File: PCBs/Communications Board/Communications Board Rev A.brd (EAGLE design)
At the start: 95.9 x 90.2 mm, 21 parts

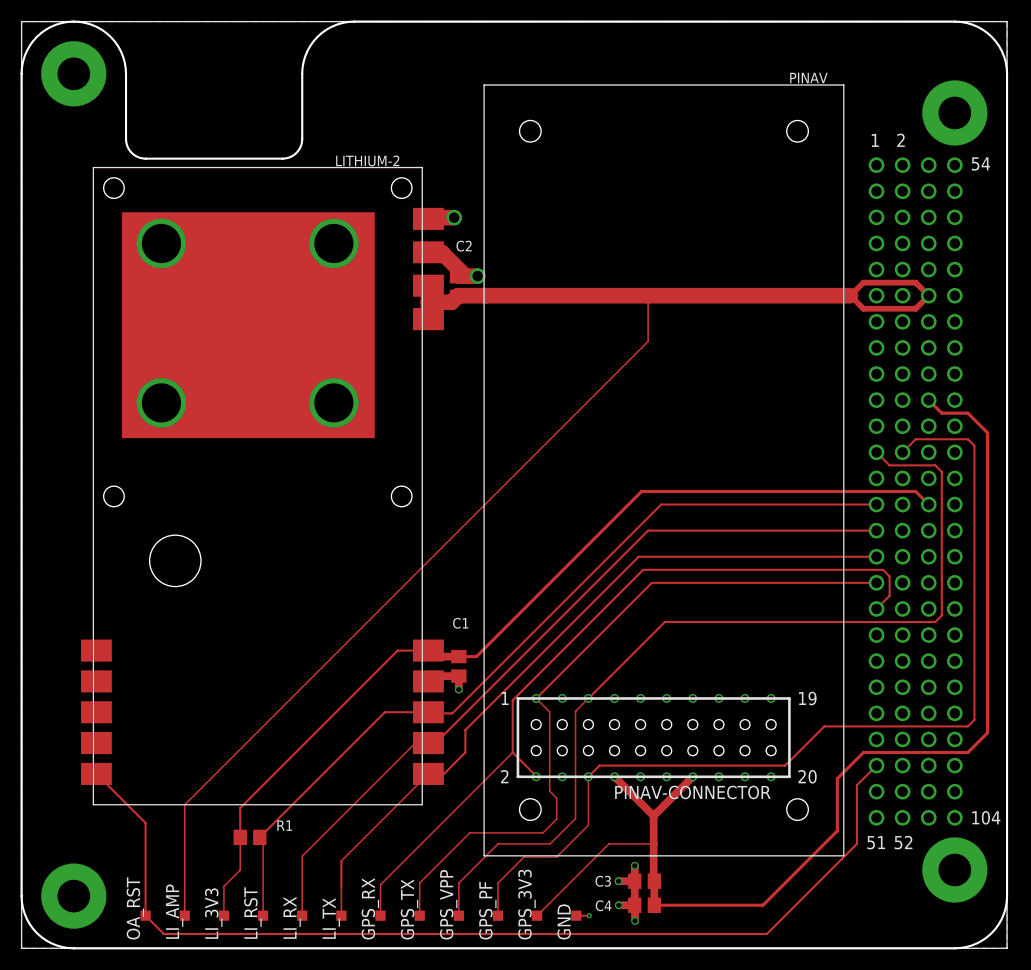
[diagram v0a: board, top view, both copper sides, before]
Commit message: Rev A2
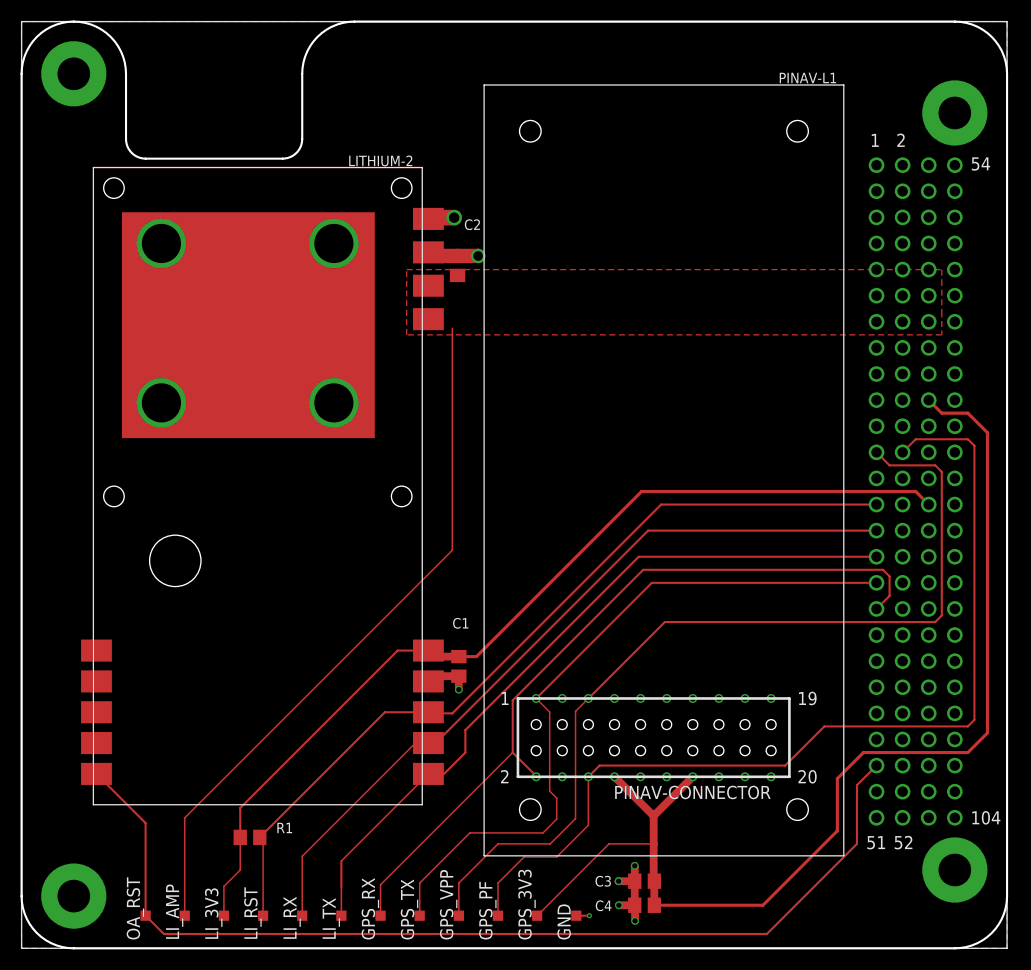
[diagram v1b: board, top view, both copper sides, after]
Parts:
- moved C2 2.03 mm to (42.4, 66.4)
- renumbered PINAV to PINAV-L1
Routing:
- net SW3: track 141.5 -> 67.9 mm
- net GND: track 23.8 -> 22.5 mm
- added copper zone on layer 1, net SW3
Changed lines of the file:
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@@
 <attribute name="VALUE" x="41.275" y="29.845" size="1.016" layer="27"/>
 </element>
-<element name="C2" library="resistor" library_urn="urn:adsk.eagle:library:348" package="C0805" package3d_urn="urn:adsk.eagle:package:23617/2" value="47uF" x="42.418" y="64.389" smashed="yes" rot="R90">
-<attribute name="NAME" x="43.9166" y="68.834" size="1.016" layer="25" rot="R180"/>
-<attribute name="VALUE" x="44.7548" y="67.564" size="1.016" layer="27" rot="R180"/>
+<element name="C2" library="resistor" library_urn="urn:adsk.eagle:library:348" package="C0805" package3d_urn="urn:adsk.eagle:package:23617/2" value="47uF" x="42.418" y="66.421" smashed="yes" rot="R90">
+<attribute name="NAME" x="44.7294" y="70.9168" size="1.016" layer="25" rot="R180"/>
+<attribute name="VALUE" x="44.7548" y="69.596" size="1.016" layer="27" rot="R180"/>
 </element>
 <element name="C3" library="resistor" library_urn="urn:adsk.eagle:library:348" package="C0805" package3d_urn="urn:adsk.eagle:package:23617/2" value="0.1uF" x="60.613" y="6.531" smashed="yes" rot="R180">
@@
 <attribute name="VALUE" x="62.8564" y="3.6068" size="1.016" layer="27"/>
 </element>
-<element name="PINAV" library="Cubesat" package="PINAV-L1" value="" x="80" y="84" smashed="yes" rot="R180">
-<attribute name="NAME" x="74.6606" y="84.1734" size="1.016" layer="25"/>
+<element name="PINAV-L1" library="Cubesat" package="PINAV-L1" value="" x="80" y="84" smashed="yes" rot="R180">
+<attribute name="NAME" x="73.6446" y="84.1734" size="1.016" layer="25"/>
 </element>
 <element name="U$1" library="Cubesat" package="PC104_NO_DIMENSION" value="PC104_NO_DIMENSION" x="0" y="0"/>
@@
 </element>
 <element name="LITHIUM-2" library="Cubesat" package="LI-2" value="LI-2" x="6.985" y="13.97" smashed="yes">
-<attribute name="NAME" x="30.48" y="76.105" size="1.016" layer="25"/>
+<attribute name="NAME" x="31.75" y="76.105" size="1.016" layer="25"/>
 </element>
 <element name="LI_RST" library="testpad" library_urn="urn:adsk.eagle:library:385" package="TP10SQ" package3d_urn="urn:adsk.eagle:package:27962/1" value="TPSQTP10SQ" x="23.495" y="3.175" smashed="yes" rot="R90">
@@
 </element>
 <element name="R1" library="resistor" library_urn="urn:adsk.eagle:library:348" package="R0805" package3d_urn="urn:adsk.eagle:package:23553/2" value="47k" x="22.225" y="10.795" smashed="yes">
-<attribute name="NAME" x="24.765" y="11.43" size="1.016" layer="25"/>
-<attribute name="VALUE" x="24.765" y="9.525" size="1.016" layer="27"/>
+<attribute name="NAME" x="24.765" y="11.2014" size="1.016" layer="25"/>
+<attribute name="VALUE" x="24.765" y="9.8298" size="1.016" layer="27"/>
 </element>
 </elements>
@@
 <signal name="SW3">
 <contactref element="C2" pad="1"/>
-<wire x1="81.915" y1="64.77" x2="80.645" y2="63.5" width="0.5588" layer="1"/>
-<wire x1="81.915" y1="64.77" x2="86.995" y2="64.77" width="0.5588" layer="1"/>
-<wire x1="81.915" y1="62.23" x2="80.645" y2="63.5" width="0.5588" layer="1"/>
-<wire x1="81.915" y1="62.23" x2="86.995" y2="62.23" width="0.5588" layer="1"/>
-<wire x1="80.645" y1="63.5" x2="60.96" y2="63.5" width="1.524" layer="1"/>
 <contactref element="U$1" pad="63"/>
-<wire x1="86.995" y1="64.77" x2="88.265" y2="63.5" width="0.5588" layer="1"/>
-<wire x1="86.995" y1="62.23" x2="88.265" y2="63.5" width="0.5588" layer="1"/>
 <contactref element="LI_AMP" pad="TP"/>
-<wire x1="60.96" y1="63.5" x2="60.96" y2="59.055" width="0.1524" layer="1"/>
-<wire x1="15.875" y1="13.97" x2="15.875" y2="3.175" width="0.1524" layer="1"/>
-<wire x1="60.96" y1="59.055" x2="15.875" y2="13.97" width="0.1524" layer="1"/>
-<wire x1="45.151" y1="63.5" x2="60.96" y2="63.5" width="1.524" layer="1"/>
 <contactref element="LITHIUM-2" pad="V_AMP2"/>
 <contactref element="LITHIUM-2" pad="V_AMP1"/>
-<wire x1="39.784" y1="61.021" x2="39.585" y2="61.22" width="1.524" layer="1"/>
-<wire x1="45.151" y1="63.5" x2="45.151" y2="63.5" width="1.524" layer="1"/>
-<wire x1="42.418" y1="63.439" x2="42.479" y2="63.5" width="1.524" layer="1"/>
-<wire x1="42.479" y1="63.5" x2="45.151" y2="63.5" width="1.524" layer="1"/>
-<wire x1="39.585" y1="64.47" x2="39.585" y2="62.865" width="1.524" layer="1"/>
-<wire x1="39.585" y1="62.865" x2="39.585" y2="61.22" width="1.524" layer="1"/>
-<wire x1="39.585" y1="61.22" x2="39.784" y2="61.021" width="1.524" layer="1"/>
-<wire x1="39.585" y1="62.865" x2="41.844" y2="62.865" width="1.524" layer="1"/>
-<wire x1="41.844" y1="62.865" x2="42.418" y2="63.439" width="1.524" layer="1"/>
+<polygon width="0.1524" layer="1" thermals="no">
+<vertex x="89.535" y="65.024"/>
+<vertex x="89.535" y="61.976"/>
+<vertex x="89.535" y="59.69"/>
+<vertex x="37.465" y="59.69"/>
+<vertex x="37.465" y="66.04"/>
+<vertex x="89.535" y="66.04"/>
+</polygon>
+<wire x1="15.875" y1="3.175" x2="15.875" y2="12.7" width="0.1524" layer="1"/>
+<wire x1="15.875" y1="12.7" x2="41.91" y2="38.735" width="0.1524" layer="1"/>
+<wire x1="41.91" y1="38.735" x2="41.91" y2="60.325" width="0.1524" layer="1"/>
 </signal>
 <signal name="OA_RESET">
@@
 <wire x1="39.585" y1="25.97" x2="39.52" y2="26.035" width="0.762" layer="1"/>
 <wire x1="40.037" y1="67.72" x2="39.585" y2="67.72" width="1.524" layer="1"/>
-<wire x1="42.484" y1="65.405" x2="43.18" y2="65.405" width="1.524" layer="1"/>
-<via x="44.3738" y="65.405" extent="1-16" drill="1.016"/>
-<wire x1="43.18" y1="65.405" x2="44.3738" y2="65.405" width="1.524" layer="1"/>
+<via x="44.4246" y="67.3608" extent="1-16" drill="0.9398"/>
 <wire x1="42.545" y1="26.482" x2="40.097" y2="26.482" width="0.762" layer="1"/>
 <wire x1="40.097" y1="26.482" x2="39.585" y2="25.97" width="0.762" layer="1"/>
 <wire x1="42.545" y1="26.482" x2="42.545" y2="25.1714" width="0.762" layer="1"/>
 <via x="42.545" y="25.1714" extent="1-16" drill="0.508"/>
-<wire x1="39.585" y1="67.72" x2="40.865" y2="67.72" width="1.524" layer="1"/>
-<wire x1="40.865" y1="67.72" x2="43.18" y2="65.405" width="1.524" layer="1"/>
-<wire x1="42.484" y1="65.405" x2="42.418" y2="65.339" width="0" layer="19" extent="1-1"/>
-<wire x1="22.065" y1="60.63" x2="30.385" y2="53.07" width="0" layer="19" extent="1-1"/>
+<wire x1="39.585" y1="67.72" x2="39.585" y2="67.371" width="1.397" layer="1"/>
+<wire x1="39.585" y1="67.371" x2="42.418" y2="67.371" width="1.397" layer="1"/>
+<wire x1="42.418" y1="67.371" x2="44.4144" y2="67.371" width="1.397" layer="1"/>
+<wire x1="30.385" y1="53.07" x2="22.065" y2="60.63" width="0" layer="19" extent="1-1"/>
+<wire x1="44.4144" y1="67.371" x2="44.4246" y2="67.3608" width="1.397" layer="1"/>
 </signal>
 <signal name="GPS_TX">
